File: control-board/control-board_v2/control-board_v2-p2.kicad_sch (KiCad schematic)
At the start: 30 parts, among them Q1 NMOS, Q2 NMOS, U2 Opamp_Dual, U3 ADS1118, U4 Opamp_Dual

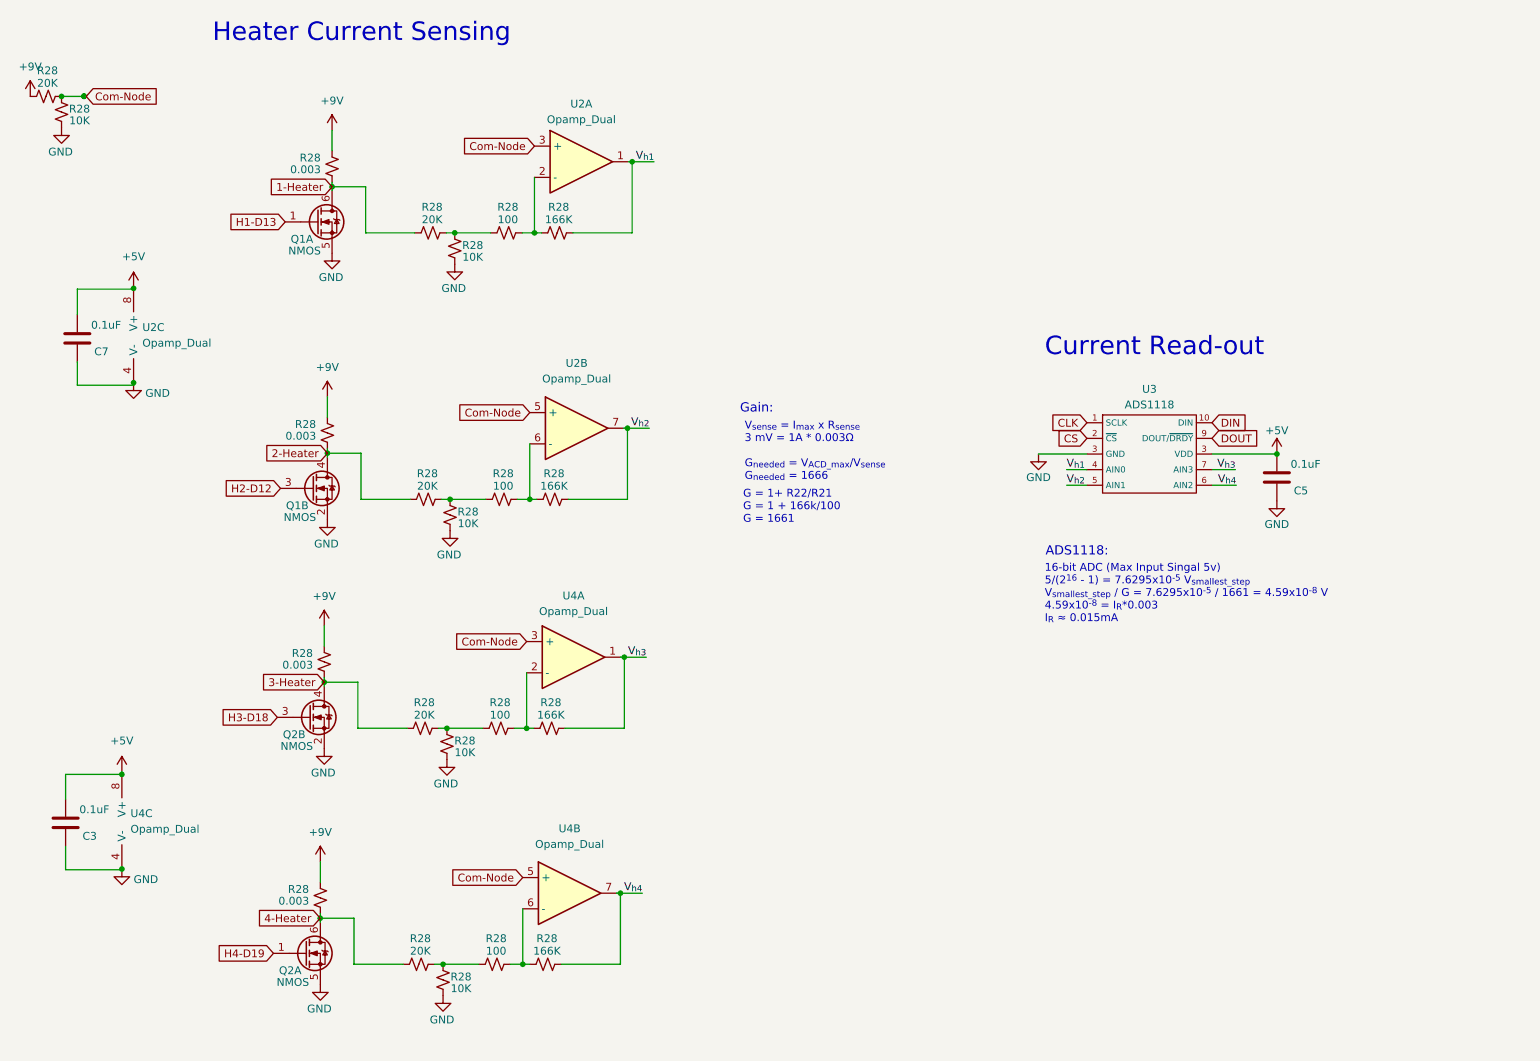
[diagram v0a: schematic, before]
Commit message: v3 with relay
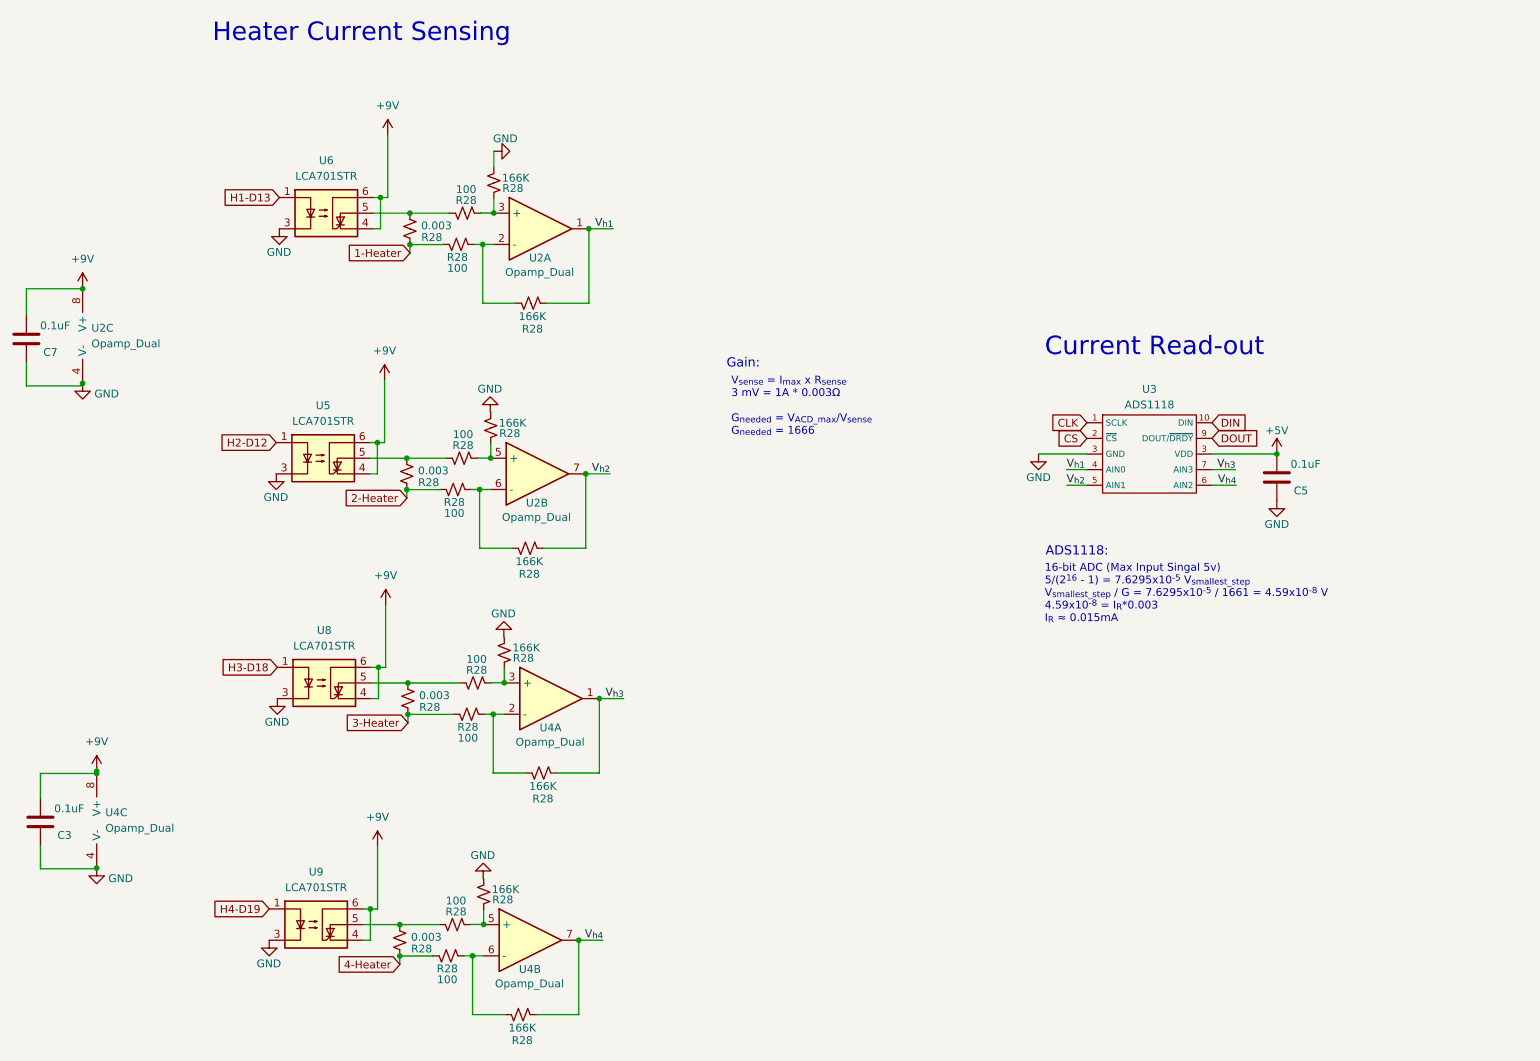
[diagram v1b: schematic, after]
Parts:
- removed Q1, Q2: NMOS, Package_TO_SOT_SMD:SOT-23-6, symbol Device:Q_Dual_NMOS_G1S2G2D2S1D1
- removed R28 (x5): 20K, Resistor_SMD:R_0805_2012Metric, symbol Device:R_Small_US
- removed R28 (x3): 100, Resistor_SMD:R_0805_2012Metric, symbol Device:R_Small_US
- removed R28 (x4): 0.003, Resistor_SMD:R_2512_6332Metric, symbol Device:R_Small_US
- removed R28 (x5): 10K, Resistor_SMD:R_0805_2012Metric, symbol Device:R_Small_US
- removed R28 (x3): 166K, Resistor_SMD:R_0603_1608Metric, symbol Device:R_Small_US
- added R28 (x7): 100, Resistor_SMD:R_0805_2012Metric, symbol Device:R_Small_US
- added R28 (x7): 166K, Resistor_SMD:R_0805_2012Metric, symbol Device:R_Small_US
- added R28 (x4): 0.003, Resistor_SMD:R_2512_6332Metric, symbol Device:R_Small_US
- added U5, U6, U8, U9: LCA701STR, Package_SO:SOIC-6_New, symbol Relay_SolidState:TLP148G
- R28: footprint Resistor_SMD:R_0603_1608Metric -> Resistor_SMD:R_0805_2012Metric
- U2, U4: Part (none) -> LM358DR
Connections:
- net +5V: no longer C3.1, C7.1, U2.8 (V+), U4.8 (V+)
- net +9V: now also C3.1, C7.1, U2.8 (V+), U4.8 (V+), U5.4, U5.6, U6.4, U6.6, U8.4, U8.6, U9.4, U9.6
- net 1-Heater: now also R28.1, R28.2
- net 2-Heater: now also R28.1, R28.2
- net 3-Heater: now also R28.1, R28.2
- net 4-Heater: now also R28.1, R28.2
- net GND: now also R28.2, R28.2, R28.2, R28.2, U5.3, U6.3, U8.3, U9.3
- net H1-D13: now also U6.1
- net H2-D12: now also U5.1
- net H3-D18: now also U8.1
- net H4-D19: now also U9.1
- net V_{h1}: now also R28.1; no longer R28.1
- net V_{h2}: now also R28.1
- net V_{h3}: now also R28.1
- net V_{h4}: now also R28.1
- net at R28.2: now also R28.1, U6.5
- net at U2.6 (-): now also R28.2, R28.2
- net at U4.6 (-): now also R28.2, R28.2
- net at U4.2 (-): now also R28.2, R28.2
- removed net Com-Node: U2.3 (+), U2.5 (+), U4.3 (+), U4.5 (+)
- new net: R28.1, R28.1, U4.3 (+)
- new net: R28.1, R28.2, U8.5
- new net: R28.1, R28.1, U2.5 (+)
- new net: R28.1, R28.2, U5.5
- new net: R28.1, R28.1, U4.5 (+)
- new net: R28.1, R28.1, U2.3 (+)
- new net: R28.2, R28.2, U2.2 (-)
- new net: R28.1, R28.2, U9.5
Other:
- note removed: "G = 1+ R22/R21 G = 1 + 166k/100 G = 1661"
- moved on the sheet: C3, C7, R28, U2A, U2C, U4C
